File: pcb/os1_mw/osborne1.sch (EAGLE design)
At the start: 17 parts

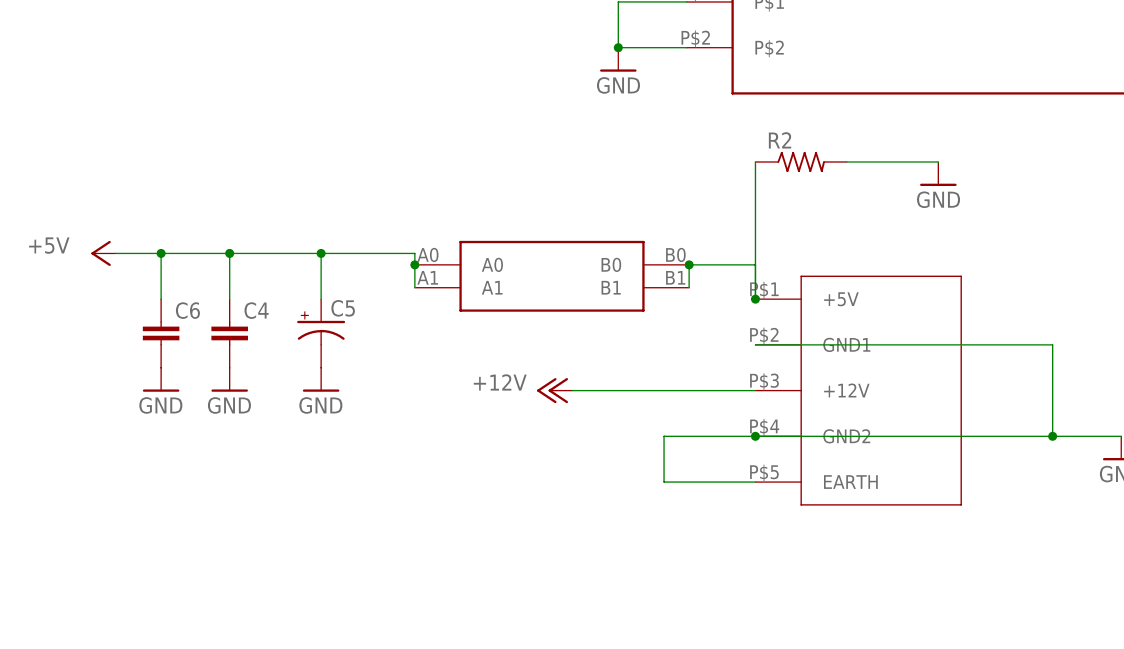
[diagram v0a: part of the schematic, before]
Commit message: updated osborne 1 pcb
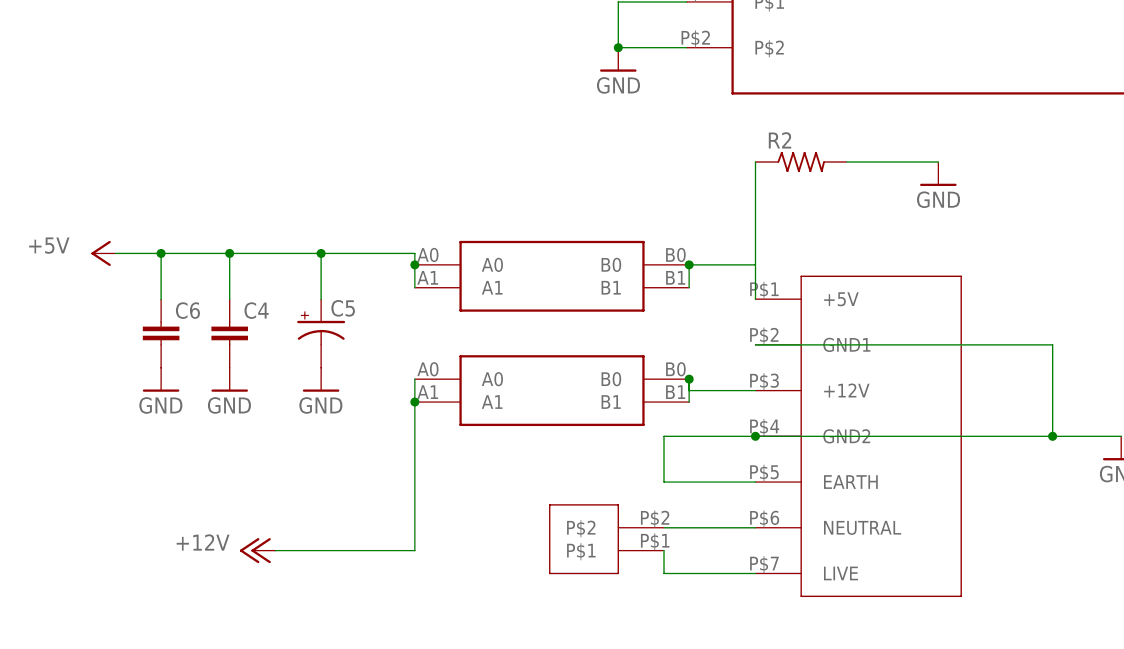
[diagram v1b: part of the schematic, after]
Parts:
- added U$3: TERM_RD50_MAINS, os1:TERM_RD50_MAINS
- added U$7: CAR_FUSE_HOLDER3IN1, atx_power_control:CAR_FUSE_HOLDER3IN1
- U$2: value TERM_RD50 -> 396_2P_LIVE; device os1:TERM_RD50 -> 396_conn:396_2P_LIVE
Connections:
- new net N$1: U$3.+12V, U$7.B0, U$7.B1
- new net N$3: U$2.P$2, U$3.NEUTRAL
- new net N$4: U$2.P$1, U$3.LIVE
- net +12V: now also U$7.A0, U$7.A1; no longer U$2.+12V
- net GND: now also U$3.EARTH, U$3.GND1, U$3.GND2; no longer U$2.EARTH, U$2.GND1, U$2.GND2
- net N$2: now also U$3.+5V; no longer U$2.+5V
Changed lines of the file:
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@@
 <parts>
 <part name="U$1" library="os1" deviceset="MEANWELL_RD50" device=""/>
-<part name="U$2" library="os1" deviceset="TERM_RD50" device=""/>
 <part name="JP2" library="pinhead" library_urn="urn:adsk.eagle:library:325" deviceset="PINHD-1X4" device="/90" package3d_urn="urn:adsk.eagle:package:22404/2"/>
 <part name="JP1" library="pinhead" library_urn="urn:adsk.eagle:library:325" deviceset="PINHD-1X4" device="/90" package3d_urn="urn:adsk.eagle:package:22404/2"/>
@@
 <part name="GND3" library="supply1" library_urn="urn:adsk.eagle:library:371" deviceset="GND" device=""/>
 <part name="GND5" library="supply1" library_urn="urn:adsk.eagle:library:371" deviceset="GND" device=""/>
+<part name="U$3" library="os1" deviceset="TERM_RD50_MAINS" device=""/>
+<part name="U$2" library="396_conn" deviceset="396_2P_LIVE" device=""/>
+<part name="U$7" library="atx_power_control" deviceset="CAR_FUSE_HOLDER" device="3IN1"/>
 </parts>
 <sheets>
@@
 <instances>
 <instance part="U$1" gate="G$1" x="45.72" y="38.1" smashed="yes"/>
-<instance part="U$2" gate="G$1" x="30.48" y="-25.4" smashed="yes"/>
 <instance part="JP2" gate="A" x="180.34" y="-17.78" smashed="yes">
 <attribute name="NAME" x="173.99" y="-9.525" size="1.778" layer="95"/>
@@
 <attribute name="VALUE" x="-60.96" y="-7.62" size="1.778" layer="96" rot="MR0"/>
 </instance>
-<instance part="P+3" gate="1" x="-7.62" y="-22.86" smashed="yes" rot="MR270">
-<attribute name="VALUE" x="-10.16" y="-22.86" size="1.778" layer="96" rot="MR0"/>
+<instance part="P+3" gate="1" x="-40.64" y="-40.64" smashed="yes" rot="MR270">
+<attribute name="VALUE" x="-43.18" y="-40.64" size="1.778" layer="96" rot="MR0"/>
 </instance>
 <instance part="GND4" gate="1" x="55.88" y="-30.48" smashed="yes" rot="MR0">
@@
 <attribute name="VALUE" x="2.54" y="10.16" size="1.778" layer="96" rot="MR0"/>
 </instance>
+<instance part="U$3" gate="G$1" x="30.48" y="-25.4" smashed="yes"/>
+<instance part="U$2" gate="G$1" x="0" y="-40.64" smashed="yes" rot="R180"/>
+<instance part="U$7" gate="G$1" x="-7.62" y="-22.86" smashed="yes"/>
 </instances>
 <busses>
@@
 <segment>
 <pinref part="GND4" gate="1" pin="GND"/>
-<pinref part="U$2" gate="G$1" pin="GND2"/>
+<wire x1="5.08" y1="-27.94" x2="15.24" y2="-27.94" width="0.1524" layer="91"/>
 <wire x1="15.24" y1="-27.94" x2="48.26" y2="-27.94" width="0.1524" layer="91"/>
 <wire x1="48.26" y1="-27.94" x2="55.88" y2="-27.94" width="0.1524" layer="91"/>
-<pinref part="U$2" gate="G$1" pin="GND1"/>
 <wire x1="15.24" y1="-17.78" x2="48.26" y2="-17.78" width="0.1524" layer="91"/>
 <wire x1="48.26" y1="-17.78" x2="48.26" y2="-27.94" width="0.1524" layer="91"/>
 <junction x="48.26" y="-27.94"/>
-<wire x1="15.24" y1="-27.94" x2="5.08" y2="-27.94" width="0.1524" layer="91"/>
 <wire x1="5.08" y1="-27.94" x2="5.08" y2="-33.02" width="0.1524" layer="91"/>
+<wire x1="5.08" y1="-33.02" x2="15.24" y2="-33.02" width="0.1524" layer="91"/>
+<pinref part="U$3" gate="G$1" pin="GND1"/>
+<pinref part="U$3" gate="G$1" pin="GND2"/>
 <junction x="15.24" y="-27.94"/>
-<pinref part="U$2" gate="G$1" pin="EARTH"/>
-<wire x1="5.08" y1="-33.02" x2="15.24" y2="-33.02" width="0.1524" layer="91"/>
+<pinref part="U$3" gate="G$1" pin="EARTH"/>
 </segment>
 <segment>
@@
 <net name="+12V" class="0">
 <segment>
-<pinref part="U$2" gate="G$1" pin="+12V"/>
-<pinref part="P+3" gate="1" pin="+12V"/>
-<wire x1="15.24" y1="-22.86" x2="-5.08" y2="-22.86" width="0.1524" layer="91"/>
-</segment>
-<segment>
 <pinref part="JP2" gate="A" pin="2"/>
 <pinref part="JP1" gate="A" pin="2"/>
@@
 <wire x1="172.72" y1="22.86" x2="200.66" y2="22.86" width="0.1524" layer="91"/>
 </segment>
+<segment>
+<pinref part="U$7" gate="G$1" pin="A1"/>
+<pinref part="U$7" gate="G$1" pin="A0"/>
+<wire x1="-22.606" y1="-24.13" x2="-22.606" y2="-21.59" width="0.1524" layer="91"/>
+<pinref part="P+3" gate="1" pin="+12V"/>
+<wire x1="-22.606" y1="-24.13" x2="-22.606" y2="-40.64" width="0.1524" layer="91"/>
+<wire x1="-22.606" y1="-40.64" x2="-38.1" y2="-40.64" width="0.1524" layer="91"/>
+<junction x="-22.606" y="-24.13"/>
+</segment>
 </net>
 <net name="N$2" class="0">
@@
 <pinref part="U$9" gate="G$1" pin="B0"/>
 <wire x1="7.874" y1="-11.43" x2="7.874" y2="-8.89" width="0.1524" layer="91"/>
-<pinref part="U$2" gate="G$1" pin="+5V"/>
 <wire x1="15.24" y1="-12.7" x2="15.24" y2="-8.89" width="0.1524" layer="91"/>
 <wire x1="15.24" y1="-8.89" x2="7.874" y2="-8.89" width="0.1524" layer="91"/>
 <junction x="7.874" y="-8.89"/>
 <pinref part="R2" gate="G$1" pin="1"/>
-<wire x1="15.24" y1="2.54" x2="15.24" y2="-12.7" width="0.1524" layer="91"/>
-<junction x="15.24" y="-12.7"/>
+<wire x1="15.24" y1="2.54" x2="15.24" y2="-8.89" width="0.1524" layer="91"/>
+<pinref part="U$3" gate="G$1" pin="+5V"/>
 </segment>
 </net>
@@
 </segment>
 </net>
+<net name="N$1" class="0">
+<segment>
+<pinref part="U$3" gate="G$1" pin="+12V"/>
+<pinref part="U$7" gate="G$1" pin="B0"/>
+<wire x1="15.24" y1="-22.86" x2="7.874" y2="-22.86" width="0.1524" layer="91"/>
+<wire x1="7.874" y1="-22.86" x2="7.874" y2="-21.59" width="0.1524" layer="91"/>
+<pinref part="U$7" gate="G$1" pin="B1"/>
+<wire x1="7.874" y1="-24.13" x2="7.874" y2="-21.59" width="0.1524" layer="91"/>
+<junction x="7.874" y="-21.59"/>
+</segment>
+</net>
+<net name="N$3" class="0">
+<segment>
+<pinref part="U$3" gate="G$1" pin="NEUTRAL"/>
+<pinref part="U$2" gate="G$1" pin="P$2"/>
+<wire x1="15.24" y1="-38.1" x2="5.08" y2="-38.1" width="0.1524" layer="91"/>
+</segment>
+</net>
+<net name="N$4" class="0">
+<segment>
+<pinref part="U$2" gate="G$1" pin="P$1"/>
+<wire x1="5.08" y1="-40.64" x2="5.08" y2="-43.18" width="0.1524" layer="91"/>
+<pinref part="U$3" gate="G$1" pin="LIVE"/>
+<wire x1="5.08" y1="-43.18" x2="15.24" y2="-43.18" width="0.1524" layer="91"/>
+</segment>
+</net>
